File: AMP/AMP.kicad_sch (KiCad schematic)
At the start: 147 parts, among them U1 NE5532, U2 NE5532, U3 NE5532, U4 NE5532, U5 NE5532, U6 NE5532, U7 NE5532, U8 NE5532

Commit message: amp updated files
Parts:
- removed C? (x8): 100n, symbol Device:C_Small
- gave numbers to parts that had none: 111
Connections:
- net POWER_AMP_IN_L: now also U10.3 (+), U10.5 (+), U12.3 (+), U12.5 (+), U13.3 (+), U13.5 (+), U9.3 (+), U9.5 (+)
- net POWER_AMP_IN_R: now also U14.3 (+), U14.5 (+), U15.3 (+), U15.5 (+), U17.3 (+), U17.5 (+), U18.3 (+), U18.5 (+)
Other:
- moved on the sheet: C1, C10, C11, C12, C13, C14, C15, C16, C23, C24, C25, C26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

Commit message: schematic done
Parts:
- added C37, C38: 2200u, Capacitor_THT:CP_Radial_D12.5mm_P5.00mm, symbol Device:C_Polarized_Small
- added R65, R67: 10, Resistor_SMD:R_0603_1608Metric, symbol Device:R_Small
- added R66, R68: 10k, Resistor_SMD:R_1206_3216Metric, symbol Device:R_Small
- C1, C4: footprint (none) -> Capacitor_THT:CP_Radial_D6.3mm_P2.50mm; LCSC (none) -> C2831780
- C10, C11, C12, C23, C24, C9: footprint (none) -> Resistor_SMD:R_0603_1608Metric; LCSC (none) -> C14858
- C13, C14, C15, C16, C21, C22, C26, C27, C28, C29, C30, C32, C33, C34, C35, C36, C7, C8: footprint (none) -> Resistor_SMD:R_0603_1608Metric; LCSC (none) -> C14663
- C17, C18: footprint (none) -> Capacitor_THT:C_Rect_L24.0mm_W12.8mm_P22.50mm_MKT; LCSC (none) -> C3019077
- C19, C20: footprint (none) -> Capacitor_SMD:C_0201_0603Metric; LCSC (none) -> C1588
- C2, C3, C5, C6: footprint (none) -> Resistor_SMD:R_0603_1608Metric; LCSC (none) -> C96446
- C25, C31: footprint (none) -> Capacitor_THT:C_Axial_L22.0mm_D10.5mm_P27.50mm_Horizontal; LCSC (none) -> C5116053
- R1, R2, R8, R9: footprint (none) -> Resistor_THT:R_Axial_DIN0516_L15.5mm_D5.0mm_P20.32mm_Horizontal; LCSC (none) -> C714455
- R10, R7: footprint (none) -> Resistor_SMD:R_1206_3216Metric; LCSC (none) -> C706452
- R11, R12, R25, R26, R39, R40: footprint (none) -> Resistor_SMD:R_0603_1608Metric; LCSC (none) -> C445632
- R13, R14, R15, R16, R21, R22, R29, R3, R32, R4: footprint (none) -> Resistor_SMD:R_0603_1608Metric; LCSC (none) -> C110776
- R17, R18: footprint (none) -> Resistor_SMD:R_0603_1608Metric; LCSC (none) -> C307918
- R19, R20, R23, R24, R33, R34, R35, R36, R41, R42, R46, R49, R5, R57, R6, R60: footprint (none) -> Resistor_SMD:R_0603_1608Metric; LCSC (none) -> C319922
- R27, R28, R37, R38: footprint (none) -> Resistor_SMD:R_0603_1608Metric; LCSC (none) -> C375508
- R30, R31: footprint (none) -> Resistor_SMD:R_0603_1608Metric; LCSC (none) -> C217683
- R43, R54: footprint (none) -> Resistor_SMD:R_1206_3216Metric; LCSC (none) -> C406727
- R44, R45, R47, R48, R50, R51, R52, R53, R55, R56, R58, R59, R61, R62, R63, R64: footprint (none) -> Resistor_SMD:R_1206_3216Metric; LCSC (none) -> C111291
- U1, U10, U11, U12, U13, U14, U15, U16, U17, U18, U2, U3, U4, U5, U6, U7, U8, U9: footprint (none) -> AUDIO_ECAD:NE5532DR; LCSC (none) -> C7426
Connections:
- net GND: now also R66.1, R68.1
- net POWER_AMP_OUT_L: now also R65.1
- net POWER_AMP_OUT_R: now also R67.1
- new net: C37.1, R65.2
- new net: C38.1, R67.2
- new net AUDIO_OUT_L: C37.2, R66.2
- new net AUDIO_OUT_R: C38.2, R68.2
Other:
- note added: "Output Protection & Filtering (LEFT)"
- moved on the sheet: C25, C26, C27, C28, C29, C30, C31, C32, C33, C34, C35, C36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

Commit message: amp updated files
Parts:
- added J1, J3: AudioJack4, Connector_Audio:Jack_3.5mm_PJ320D_Horizontal, symbol Connector:AudioJack4
- added J2: Screw_Terminal_01x02, TerminalBlock:TerminalBlock_Altech_AK300-2_P5.00mm, symbol Connector:Screw_Terminal_01x02
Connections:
- net +15V: now also C13.1, C14.1, C15.1, C16.1, C21.1, C22.1, C26.1, C27.1, C28.1, C29.1, C30.1, C32.1, C33.1, C34.1, C35.1, C36.1, C7.1, C8.1, U1.8 (V+), U10.8 (V+), U11.8 (V+), U12.8 (V+), U13.8 (V+), U14.8 (V+), U15.8 (V+), U16.8 (V+), U17.8 (V+), U18.8 (V+), U2.8 (V+), U3.8 (V+), U4.8 (V+), U5.8 (V+), U6.8 (V+), U7.8 (V+), U8.8 (V+), U9.8 (V+), J2.1 (Pin_1)
- net AUDIO_OUT_L: now also J3.T
- net AUDIO_OUT_R: now also J3.R1
- net GND: now also C13.2, C14.2, C15.2, C16.2, C21.2, C22.2, C26.2, C27.2, C28.2, C29.2, C30.2, C32.2, C33.2, C34.2, C35.2, C36.2, C7.2, C8.2, U1.4 (V-), U10.4 (V-), U11.4 (V-), U12.4 (V-), U13.4 (V-), U14.4 (V-), U15.4 (V-), U16.4 (V-), U17.4 (V-), U18.4 (V-), U2.4 (V-), U3.4 (V-), U4.4 (V-), U5.4 (V-), U6.4 (V-), U7.4 (V-), U8.4 (V-), U9.4 (V-), J1.S, J2.2 (Pin_2), J3.S
- net LEFT_AUDIO_IN: now also J1.R1
- net RIGHT_AUDIO_IN: now also J1.T
- no-connect marks 0 -> 2
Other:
- moved on the sheet: C13, C14, C15, C16, C17, C18, C19, C20, C21, C22, C25, C26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

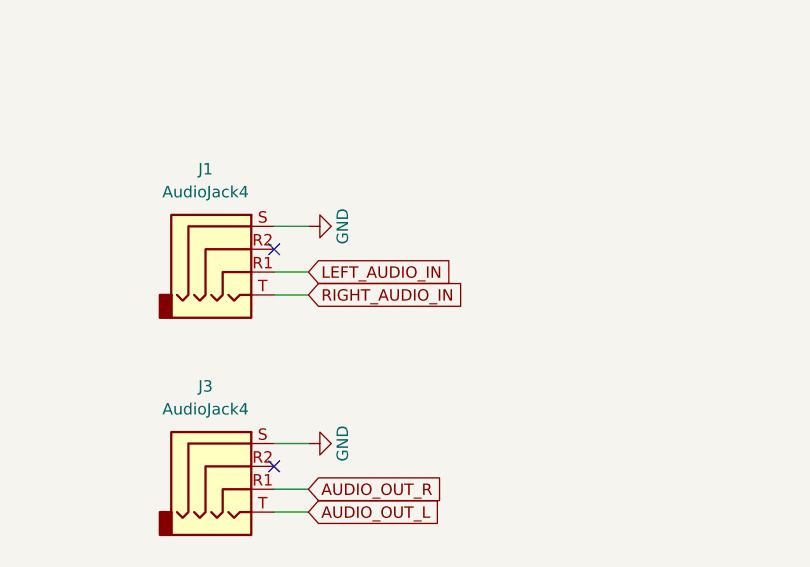
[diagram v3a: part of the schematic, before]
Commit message: pcb layout
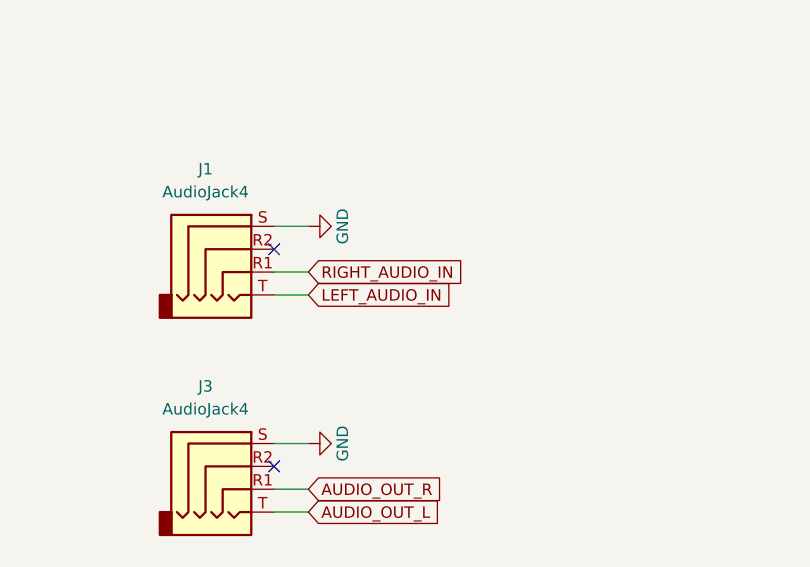
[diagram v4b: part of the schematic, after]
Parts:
- R1, R2, R8, R9: footprint Resistor_THT:R_Axial_DIN0516_L15.5mm_D5.0mm_P20.32mm_Horizontal -> Resistor_SMD:R_0603_1608Metric; LCSC C714455 -> C114662
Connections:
- net LEFT_AUDIO_IN: now also J1.T; no longer J1.R1
- net RIGHT_AUDIO_IN: now also J1.R1; no longer J1.T
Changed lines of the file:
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@@
     )
   )
-  (global_label "RIGHT_AUDIO_IN" (shape input) (at 433.07 205.74 0) (fields_autoplaced)
-    (effects (font (size 1.27 1.27)) (justify left))
-    (property "Intersheet References" "${INTERSHEET_REFS}" (id 0) (at 450.4207 205.6606 0)
-      (effects (font (size 1.27 1.27)) (justify left) hide)
-    )
-  )
   (global_label "VOL_OUT_R" (shape input) (at 557.53 50.8 0) (fields_autoplaced)
     (effects (font (size 1.27 1.27)) (justify left))
@@
     )
   )
+  (global_label "RIGHT_AUDIO_IN" (shape input) (at 433.07 203.2 0) (fields_autoplaced)
+    (effects (font (size 1.27 1.27)) (justify left))
+    (property "Intersheet References" "${INTERSHEET_REFS}" (id 0) (at 450.4207 203.1206 0)
+      (effects (font (size 1.27 1.27)) (justify left) hide)
+    )
+  )
   (global_label "POWER_AMP_OUT_L" (shape input) (at 184.15 237.49 0) (fields_autoplaced)
     (effects (font (size 1.27 1.27)) (justify left))
@@
     )
   )
+  (global_label "LEFT_AUDIO_IN" (shape input) (at 433.07 205.74 0) (fields_autoplaced)
+    (effects (font (size 1.27 1.27)) (justify left))
+    (property "Intersheet References" "${INTERSHEET_REFS}" (id 0) (at 449.2112 205.8194 0)
+      (effects (font (size 1.27 1.27)) (justify left) hide)
+    )
+  )
   (global_label "POWER_AMP_IN_L" (shape input) (at 228.6 186.69 180) (fields_autoplaced)
     (effects (font (size 1.27 1.27)) (justify right))
@@
     )
   )
-  (global_label "LEFT_AUDIO_IN" (shape input) (at 433.07 203.2 0) (fields_autoplaced)
-    (effects (font (size 1.27 1.27)) (justify left))
-    (property "Intersheet References" "${INTERSHEET_REFS}" (id 0) (at 449.2112 203.2794 0)
-      (effects (font (size 1.27 1.27)) (justify left) hide)
-    )
-  )
   (global_label "VBIAS_L" (shape input) (at 279.4 69.85 180) (fields_autoplaced)
     (effects (font (size 1.27 1.27)) (justify right))
@@
       (effects (font (size 1.27 1.27)) (justify left))
     )
-    (property "Footprint" "Resistor_THT:R_Axial_DIN0516_L15.5mm_D5.0mm_P20.32mm_Horizontal" (id 2) (at 27.94 43.18 0)
+    (property "Footprint" "Resistor_SMD:R_0603_1608Metric" (id 2) (at 27.94 43.18 0)
       (effects (font (size 1.27 1.27)) hide)
     )
-    (property "Datasheet" "~" (id 3) (at 27.94 43.18 0)
+    (property "Datasheet" "https://datasheet.lcsc.com/lcsc/2304140030_YAGEO-RC0603FR-072K2L_C114662.pdf" (id 3) (at 27.94 43.18 0)
       (effects (font (size 1.27 1.27)) hide)
     )
-    (property "LCSC" "C714455" (id 4) (at 27.94 43.18 0)
+    (property "LCSC" "C114662" (id 4) (at 27.94 43.18 0)
       (effects (font (size 1.27 1.27)) hide)
     )
@@
       (effects (font (size 1.27 1.27)) (justify left))
     )
-    (property "Footprint" "Resistor_THT:R_Axial_DIN0516_L15.5mm_D5.0mm_P20.32mm_Horizontal" (id 2) (at 116.84 43.18 0)
+    (property "Footprint" "Resistor_SMD:R_0603_1608Metric" (id 2) (at 116.84 43.18 0)
       (effects (font (size 1.27 1.27)) hide)
     )
-    (property "Datasheet" "~" (id 3) (at 116.84 43.18 0)
+    (property "Datasheet" "https://datasheet.lcsc.com/lcsc/2304140030_YAGEO-RC0603FR-072K2L_C114662.pdf" (id 3) (at 116.84 43.18 0)
       (effects (font (size 1.27 1.27)) hide)
     )
-    (property "LCSC" "C714455" (id 4) (at 116.84 43.18 0)
+    (property "LCSC" "C114662" (id 4) (at 116.84 43.18 0)
       (effects (font (size 1.27 1.27)) hide)
     )
@@
       (effects (font (size 1.27 1.27)) (justify left))
     )
-    (property "Footprint" "Resistor_THT:R_Axial_DIN0516_L15.5mm_D5.0mm_P20.32mm_Horizontal" (id 2) (at 27.94 53.34 0)
+    (property "Footprint" "Resistor_SMD:R_0603_1608Metric" (id 2) (at 27.94 53.34 0)
       (effects (font (size 1.27 1.27)) hide)
     )
-    (property "Datasheet" "~" (id 3) (at 27.94 53.34 0)
+    (property "Datasheet" "https://datasheet.lcsc.com/lcsc/2304140030_YAGEO-RC0603FR-072K2L_C114662.pdf" (id 3) (at 27.94 53.34 0)
       (effects (font (size 1.27 1.27)) hide)
     )
-    (property "LCSC" "C714455" (id 4) (at 27.94 53.34 0)
+    (property "LCSC" "C114662" (id 4) (at 27.94 53.34 0)
       (effects (font (size 1.27 1.27)) hide)
     )
@@
       (effects (font (size 1.27 1.27)) (justify left))
     )
-    (property "Footprint" "Resistor_THT:R_Axial_DIN0516_L15.5mm_D5.0mm_P20.32mm_Horizontal" (id 2) (at 116.84 53.34 0)
+    (property "Footprint" "Resistor_SMD:R_0603_1608Metric" (id 2) (at 116.84 53.34 0)
       (effects (font (size 1.27 1.27)) hide)
     )
-    (property "Datasheet" "~" (id 3) (at 116.84 53.34 0)
+    (property "Datasheet" "https://datasheet.lcsc.com/lcsc/2304140030_YAGEO-RC0603FR-072K2L_C114662.pdf" (id 3) (at 116.84 53.34 0)
       (effects (font (size 1.27 1.27)) hide)
     )
-    (property "LCSC" "C714455" (id 4) (at 116.84 53.34 0)
+    (property "LCSC" "C114662" (id 4) (at 116.84 53.34 0)
       (effects (font (size 1.27 1.27)) hide)
     )
@@
     )
     (path "/200c63d5-9f0c-4606-917d-24a8280ed9ed"
-      (reference "R1") (unit 1) (value "2.2k") (footprint "Resistor_THT:R_Axial_DIN0516_L15.5mm_D5.0mm_P20.32mm_Horizontal")
+      (reference "R1") (unit 1) (value "2.2k") (footprint "Resistor_SMD:R_0603_1608Metric")
     )
     (path "/e1a0cc3c-2cac-4d0a-abe1-d80d5486209e"
-      (reference "R2") (unit 1) (value "2.2k") (footprint "Resistor_THT:R_Axial_DIN0516_L15.5mm_D5.0mm_P20.32mm_Horizontal")
+      (reference "R2") (unit 1) (value "2.2k") (footprint "Resistor_SMD:R_0603_1608Metric")
     )
     (path "/0d0a4ca1-a81c-40e5-aa87-699cf3e69320"
@@
     )
     (path "/f6de87ba-476e-4789-9f15-f77e20cfa9a4"
-      (reference "R8") (unit 1) (value "2.2k") (footprint "Resistor_THT:R_Axial_DIN0516_L15.5mm_D5.0mm_P20.32mm_Horizontal")
+      (reference "R8") (unit 1) (value "2.2k") (footprint "Resistor_SMD:R_0603_1608Metric")
     )
     (path "/f91a8d3f-d2a2-418e-a962-86afff331ba8"
-      (reference "R9") (unit 1) (value "2.2k") (footprint "Resistor_THT:R_Axial_DIN0516_L15.5mm_D5.0mm_P20.32mm_Horizontal")
+      (reference "R9") (unit 1) (value "2.2k") (footprint "Resistor_SMD:R_0603_1608Metric")
     )
     (path "/3d156a46-95e7-451b-88f8-4f39928bd8e1"
